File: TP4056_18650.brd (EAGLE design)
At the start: 60.6 x 7 mm, 17 parts, among them X1 USB MICRO

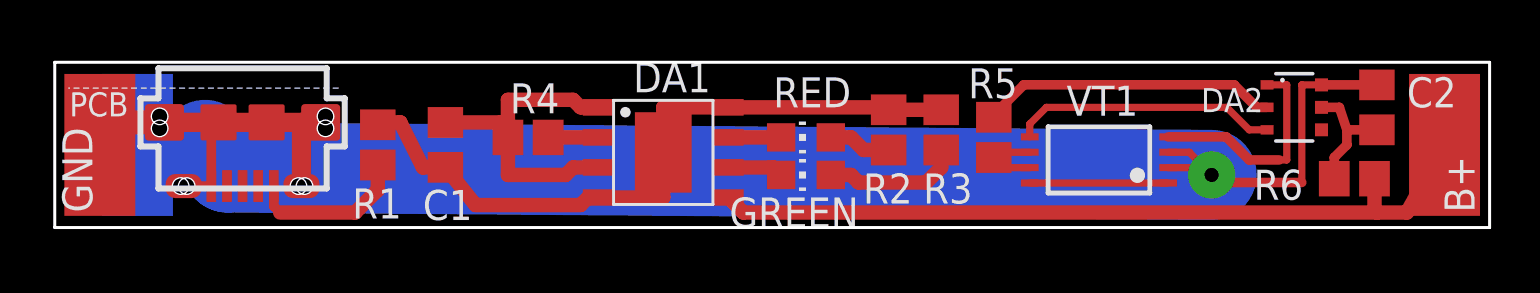
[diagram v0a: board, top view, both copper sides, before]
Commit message: .
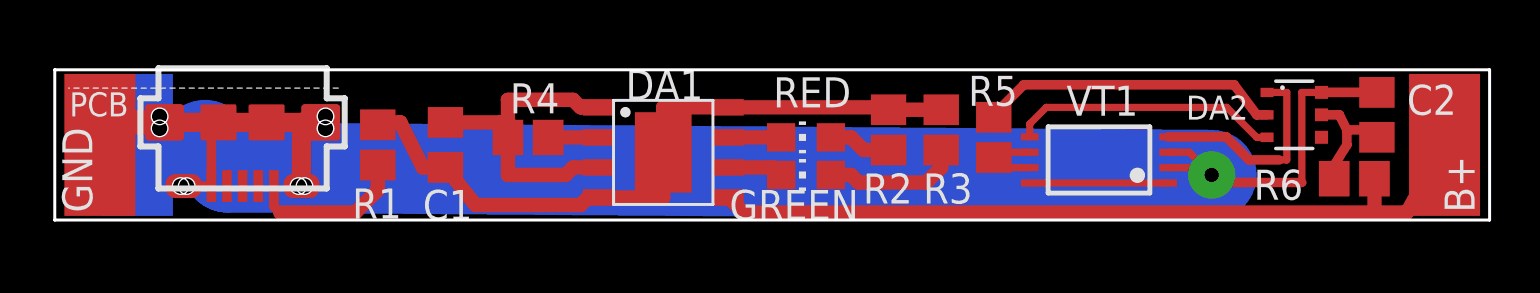
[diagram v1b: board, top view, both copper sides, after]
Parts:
- moved C2 0.32 mm to (56.2, 5.08)
- moved DA2 0.32 mm to (52.7, 5.08)
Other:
- board size 60.6 x 7 mm -> 60.6 x 6.4 mm
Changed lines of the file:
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@@
 <board>
 <plain>
-<wire x1="0.3175" y1="7.3025" x2="60.96" y2="7.3025" width="0.127" layer="20"/>
-<wire x1="60.96" y1="7.3025" x2="60.96" y2="0.3175" width="0.127" layer="20"/>
-<wire x1="60.96" y1="0.3175" x2="0.3175" y2="0.3175" width="0.127" layer="20"/>
-<wire x1="0.3175" y1="0.3175" x2="0.3175" y2="7.3025" width="0.127" layer="20"/>
-<dimension x1="0.3175" y1="11.1125" x2="60.96" y2="12.3825" x3="30.63875" y3="12.065" layer="21" dtype="horizontal"/>
-<dimension x1="-4.445" y1="7.3025" x2="-5.08" y2="0.3175" x3="-6.0325" y3="3.81" layer="21" dtype="vertical"/>
+<wire x1="0.3175" y1="6.985" x2="60.96" y2="6.985" width="0.127" layer="20"/>
+<wire x1="60.96" y1="6.985" x2="60.96" y2="0.635" width="0.127" layer="20"/>
+<wire x1="60.96" y1="0.635" x2="0.3175" y2="0.635" width="0.127" layer="20"/>
+<wire x1="0.3175" y1="0.635" x2="0.3175" y2="6.985" width="0.127" layer="20"/>
+<dimension x1="0.3175" y1="8.255" x2="60.96" y2="8.255" x3="30.63875" y3="9.2075" layer="21" dtype="horizontal"/>
+<dimension x1="-1.27" y1="6.985" x2="-1.27" y2="0.635" x3="-1.905" y3="3.81" layer="21" dtype="vertical"/>
 </plain>
 <attributes>
@@
 <elements>
 <element name="DA1" library="TP4056" package="SOP-8" value="TP4056" x="26.035" y="3.4925" smashed="yes">
-<attribute name="NAME" x="24.765" y="6.0325" size="1.27" layer="25"/>
+<attribute name="NAME" x="24.4475" y="5.715" size="1.27" layer="25"/>
 </element>
 <element name="R1" library="resistor" package="R0805" value="0.5" x="13.97" y="3.81" smashed="yes" rot="R90">
@@
 <attribute name="VALUE" x="47.7" y="6.1" size="1.27" layer="27" rot="R180"/>
 </element>
-<element name="DA2" library="DW01" package="SOT23-6" value="DW01A" x="52.705" y="5.3975" smashed="yes" rot="R270">
-<attribute name="VALUE" x="50.033" y="6.7945" size="1.016" layer="27" ratio="10" rot="R270"/>
-<attribute name="NAME" x="48.768" y="5.1945" size="1.016" layer="25" ratio="10"/>
+<element name="DA2" library="DW01" package="SOT23-6" value="DW01A" x="52.705" y="5.08" smashed="yes" rot="R270">
+<attribute name="VALUE" x="50.033" y="6.477" size="1.016" layer="27" ratio="10" rot="R270"/>
+<attribute name="NAME" x="48.133" y="4.877" size="1.016" layer="25" ratio="10"/>
 </element>
 <element name="R5" library="resistor" package="R0805" value="1k" x="40.005" y="4.1275" smashed="yes" rot="R90">
-<attribute name="NAME" x="38.9255" y="5.7785" size="1.27" layer="25"/>
+<attribute name="NAME" x="38.9255" y="5.461" size="1.27" layer="25"/>
 <attribute name="VALUE" x="42.291" y="3.3655" size="1.27" layer="27" rot="R90"/>
 </element>
-<element name="C2" library="rcl" package="C0805" value="100n" x="56.1975" y="5.3975" smashed="yes" rot="R270">
-<attribute name="NAME" x="57.4675" y="5.3975" size="1.27" layer="25"/>
-<attribute name="VALUE" x="53.6575" y="6.6675" size="1.27" layer="27" rot="R270"/>
+<element name="C2" library="rcl" package="C0805" value="100n" x="56.1975" y="5.08" smashed="yes" rot="R270">
+<attribute name="NAME" x="57.4675" y="5.08" size="1.27" layer="25"/>
+<attribute name="VALUE" x="53.6575" y="6.35" size="1.27" layer="27" rot="R270"/>
 </element>
 <element name="R6" library="resistor" package="R0805" value="100" x="55.245" y="2.38125" smashed="yes">
@@
 </element>
 <element name="GREEN" library="led" package="CHIP-LED0805" value="" x="32.0675" y="2.54" smashed="yes" rot="R90">
-<attribute name="NAME" x="34.29" y="1.5875" size="1.27" layer="25" rot="R180"/>
+<attribute name="NAME" x="34.29" y="1.905" size="1.27" layer="25" rot="R180"/>
 <attribute name="VALUE" x="33.3375" y="5.08" size="1.27" layer="27" rot="R180"/>
 </element>
@@
 <wire x1="41.525" y1="4.695" x2="42.2275" y2="5.3975" width="0.3048" layer="1"/>
 <wire x1="42.2275" y1="5.3975" x2="49.8475" y2="5.3975" width="0.3048" layer="1"/>
-<wire x1="49.8475" y1="5.3975" x2="50.7975" y2="4.4475" width="0.3048" layer="1"/>
-<wire x1="50.7975" y1="4.4475" x2="51.555" y2="4.4475" width="0.3048" layer="1"/>
+<wire x1="49.8475" y1="5.3975" x2="51.115" y2="4.13" width="0.3048" layer="1"/>
+<wire x1="51.115" y1="4.13" x2="51.555" y2="4.13" width="0.3048" layer="1"/>
 </signal>
 <signal name="N$4">
@@
 <wire x1="50.8" y1="3.175" x2="52.07" y2="3.175" width="0.4064" layer="1"/>
 <wire x1="52.07" y1="3.175" x2="52.3875" y2="3.175" width="0.3048" layer="1"/>
-<wire x1="52.3875" y1="3.175" x2="52.3875" y2="6.3475" width="0.3048" layer="1"/>
-<wire x1="52.3875" y1="6.3475" x2="51.555" y2="6.3475" width="0.3048" layer="1"/>
+<wire x1="52.3875" y1="3.175" x2="52.3875" y2="6.03" width="0.3048" layer="1"/>
+<wire x1="52.3875" y1="6.03" x2="51.555" y2="6.03" width="0.3048" layer="1"/>
 </signal>
 <signal name="B-">
@@
 <wire x1="7.62" y1="2.8575" x2="6.6675" y2="3.81" width="3.81" layer="16"/>
 <wire x1="6.6675" y1="3.81" x2="3.81" y2="3.81" width="2.1844" layer="16"/>
-<wire x1="53.855" y1="6.3475" x2="56.1975" y2="6.3475" width="0.4064" layer="1"/>
+<wire x1="53.855" y1="6.03" x2="56.1975" y2="6.03" width="0.4064" layer="1"/>
 <wire x1="49.2125" y1="2.54" x2="49.2125" y2="2.2225" width="0.4064" layer="1"/>
 <wire x1="49.2125" y1="2.2225" x2="53.0225" y2="2.2225" width="0.4064" layer="1"/>
-<wire x1="53.0225" y1="2.2225" x2="53.0225" y2="6.3475" width="0.3048" layer="1"/>
-<wire x1="53.0225" y1="6.3475" x2="53.855" y2="6.3475" width="0.3048" layer="1"/>
+<wire x1="53.0225" y1="2.2225" x2="53.0225" y2="6.03" width="0.3048" layer="1"/>
+<wire x1="53.0225" y1="6.03" x2="53.855" y2="6.03" width="0.3048" layer="1"/>
 </signal>
 <signal name="N$6">
@@
 <wire x1="40.005" y1="5.08" x2="41.275" y2="6.35" width="0.4064" layer="1"/>
 <wire x1="41.275" y1="6.35" x2="50.165" y2="6.35" width="0.4064" layer="1"/>
-<wire x1="50.165" y1="6.35" x2="51.1175" y2="5.3975" width="0.4064" layer="1"/>
-<wire x1="51.1175" y1="5.3975" x2="51.555" y2="5.3975" width="0.4064" layer="1"/>
+<wire x1="50.165" y1="6.35" x2="51.1175" y2="5.08" width="0.4064" layer="1"/>
+<wire x1="51.1175" y1="5.08" x2="51.555" y2="5.08" width="0.4064" layer="1"/>
 </signal>
 <signal name="N$8">
@@
 <contactref element="C2" pad="2"/>
 <contactref element="R6" pad="1"/>
-<wire x1="54.9275" y1="4.445" x2="54.61" y2="5.3975" width="0.4064" layer="1"/>
-<wire x1="54.61" y1="5.3975" x2="53.855" y2="5.3975" width="0.4064" layer="1"/>
+<wire x1="54.9275" y1="4.445" x2="54.61" y2="5.08" width="0.4064" layer="1"/>
+<wire x1="54.61" y1="5.08" x2="53.855" y2="5.08" width="0.4064" layer="1"/>
 <wire x1="54.9275" y1="4.445" x2="56.195" y2="4.445" width="0.4064" layer="1"/>
-<wire x1="56.195" y1="4.445" x2="56.1975" y2="4.4475" width="0.4064" layer="1"/>
-<wire x1="54.395" y1="2.38125" x2="54.395" y2="3.2775" width="0.4064" layer="1"/>
-<wire x1="54.395" y1="3.2775" x2="54.9275" y2="3.81" width="0.4064" layer="1"/>
+<wire x1="56.195" y1="4.445" x2="56.1975" y2="4.13" width="0.4064" layer="1"/>
+<wire x1="54.395" y1="2.38125" x2="54.395" y2="2.96" width="0.4064" layer="1"/>
+<wire x1="54.395" y1="2.96" x2="54.9275" y2="3.81" width="0.4064" layer="1"/>
 <wire x1="54.9275" y1="3.81" x2="54.9275" y2="4.445" width="0.4064" layer="1"/>
 </signal>
